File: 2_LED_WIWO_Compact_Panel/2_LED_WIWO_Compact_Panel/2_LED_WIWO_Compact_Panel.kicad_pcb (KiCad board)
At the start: 2 copper layers, 77.5 x 56.5 mm, 77 parts, among them J3 Screw_Terminal_01x03, J4 Screw_Terminal_01x03, Q1 AO3400A, U1 AP2210N-5.0TRG1, U2 XL1509, U3 NE555DR-EV, U4 NE555DR-EV, U5 MP24833-AGN-Z, U6 MP24833-AGN-Z

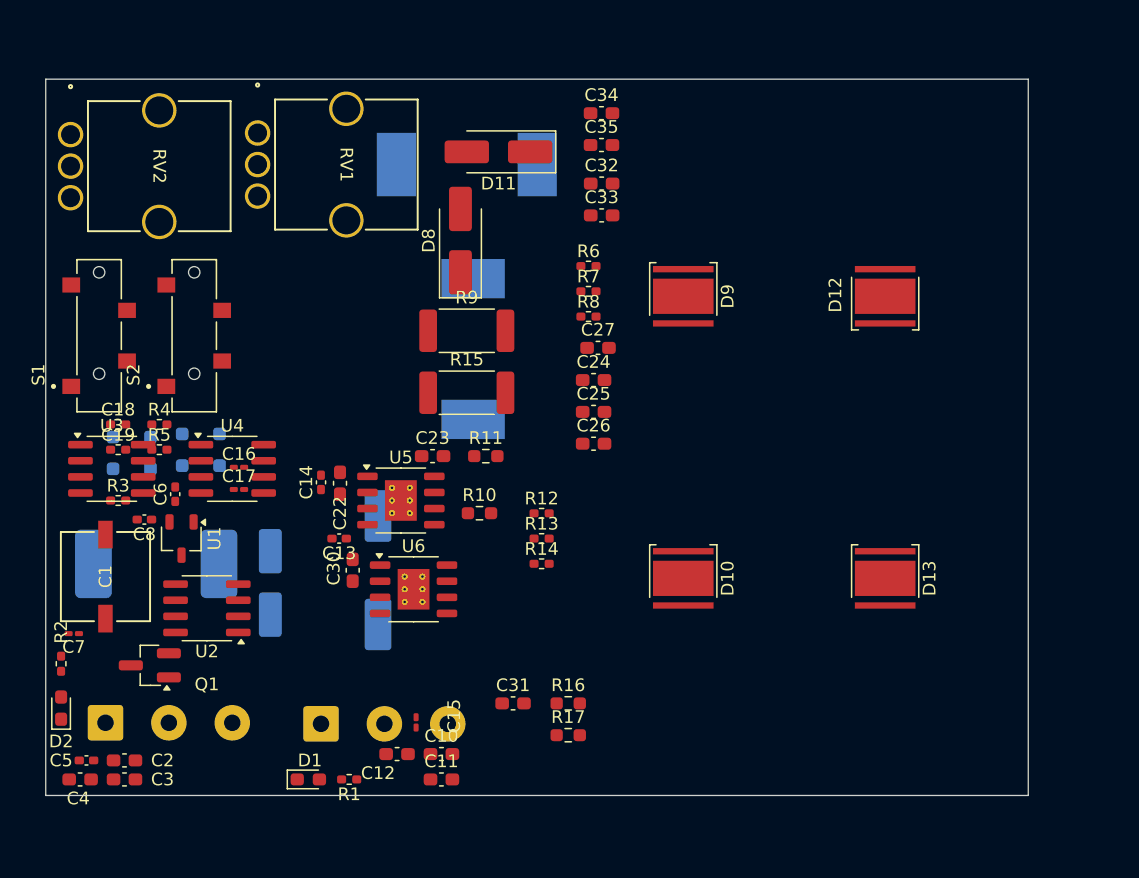
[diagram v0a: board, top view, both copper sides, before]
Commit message: v1 route done
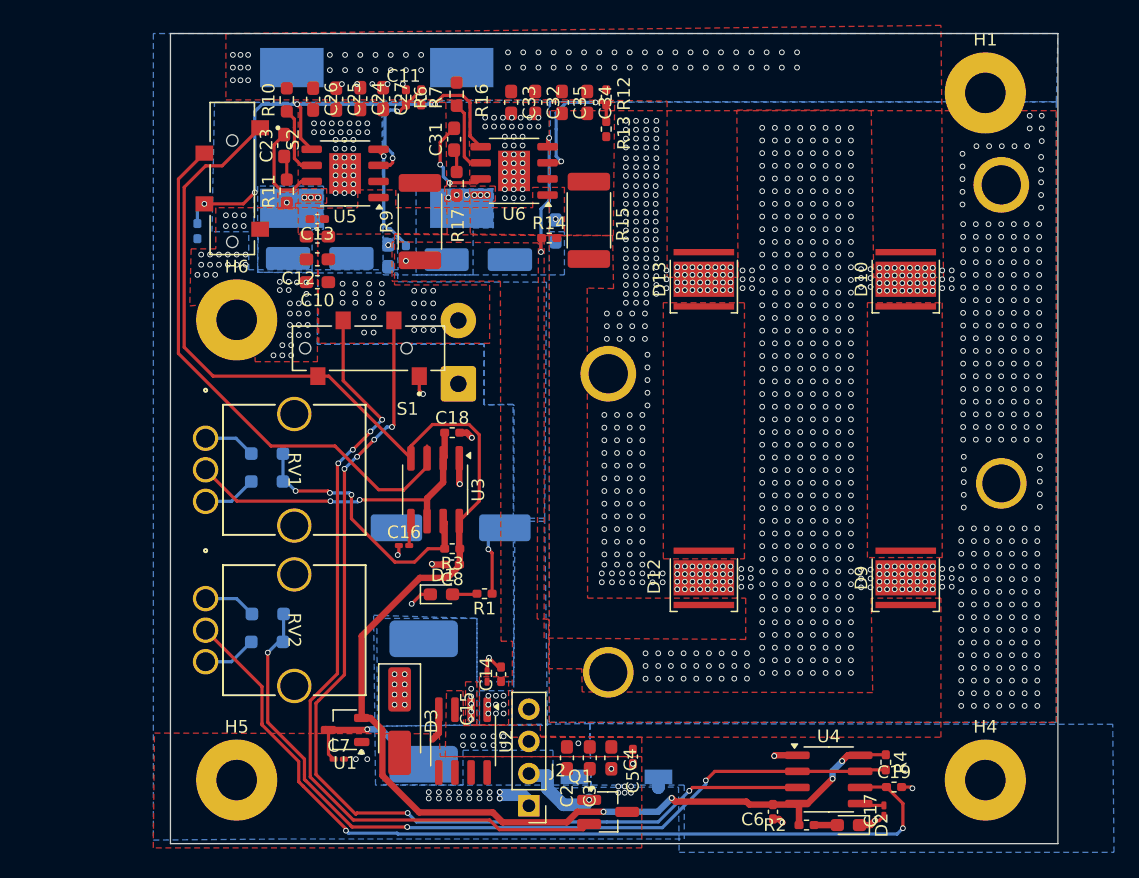
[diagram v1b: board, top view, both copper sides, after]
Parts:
- removed J3, J4: Screw_Terminal_01x03, TerminalBlock:TerminalBlock_MaiXu_MX126-5.0-03P_1x03_P5.00mm
- added E1: ~, heatsinks:small_heatsink, B.Cu at (183.7, 71.5)
- added E2: ~, heatsinks:small_heatsink, B.Cu at (183.7, 95.1)
- added H1: MountingHole_Pad, MountingHole:MountingHole_3.2mm_M3_Pad, F.Cu at (197.9, 56.9)
- added H4: MountingHole_Pad, MountingHole:MountingHole_3.2mm_M3_Pad, F.Cu at (197.9, 111.0)
- added H5: MountingHole_Pad, MountingHole:MountingHole_3.2mm_M3_Pad, F.Cu at (138.8, 111.0)
- added H6: MountingHole_Pad, MountingHole:MountingHole_3.2mm_M3_Pad, F.Cu at (138.8, 74.8)
- added J1: Screw_Terminal_01x02, TerminalBlock:TerminalBlock_MaiXu_MX126-5.0-02P_1x02_P5.00mm, B.Cu at (156.3, 79.8)
- added J2: Conn_01x04_Pin, Connector_PinHeader_2.54mm:PinHeader_1x04_P2.54mm_Vertical, F.Cu at (161.9, 113.1)
- C1, C22, C30, D11, D8, R5, R8: moved to B.Cu
- D3: moved to F.Cu
- moved C19 66.7 mm to (190.7, 111.6)
- moved R4 63.2 mm to (190.1, 109.7), turned to -90 degrees
- moved D2 62.8 mm to (187.1, 114.6), turned to 180 degrees
- moved R2 60.2 mm to (183.8, 114.6), turned to 0 degrees
- moved C17 56.8 mm to (189.9, 113.5), turned to 90 degrees
- moved C6 53.4 mm to (181.2, 113.5), turned to -90 degrees
- moved U4 53.0 mm to (185.6, 111.0)
- moved R16 48.8 mm to (156.2, 57.0), turned to 90 degrees
- moved C31 44.7 mm to (156.0, 60.5), turned to 90 degrees
- moved R17 44.4 mm to (156.2, 64.0), turned to 90 degrees
- moved C11 43.9 mm to (145.2, 68.2), turned to 180 degrees
- moved C1 43.3 mm to (168.8, 110.8), turned to 0 degrees
- moved C5 43.1 mm to (170.1, 109.2), turned to -90 degrees
- moved C4 41.9 mm to (168.4, 109.3), turned to -90 degrees
- moved C12 39.5 mm to (145.2, 70.0)
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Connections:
- C18 pad 1: /TR_THR -> /LED_TR_THR
- C19 pad 1: /TR_THR -> /FAN_TR_THR
- C22 pad 2: PGND -> PGND_1
- C24 pad 2: PGND -> PGND_1
- C25 pad 2: PGND -> PGND_1
- C26 pad 2: PGND -> PGND_1
- C27 pad 2: PGND -> PGND_1
- C30 pad 2: PGND -> PGND_2
- C32 pad 2: PGND -> PGND_2
- C33 pad 2: PGND -> PGND_2
- C34 pad 2: PGND -> PGND_2
- C35 pad 2: PGND -> PGND_2
- D11 pad 2: PGND -> PGND_2
- D4 pad 2: /DIS -> /LED_DIS
- D5 pad 2: /DIS -> /FAN_DIS
- D6 pad 1: /DIS -> /LED_DIS
- D7 pad 1: /DIS -> /FAN_DIS
- D8 pad 2: PGND -> PGND_1
- R13 pad 2: PGND -> PGND_2
- R15 pad 2: PGND -> PGND_2
- R3 pad 2: /DIS -> /LED_DIS
- R4 pad 2: /DIS -> /FAN_DIS
- R7 pad 2: PGND -> PGND_1
- R9 pad 2: PGND -> PGND_1
- RV1 pad 2: /TR_THR -> /LED_TR_THR
- RV2 pad 2: /TR_THR -> /FAN_TR_THR
- U3 pad 2: /TR_THR -> /LED_TR_THR
- U3 pad 6: /TR_THR -> /LED_TR_THR
- U3 pad 7: /DIS -> /LED_DIS
- U4 pad 2: /TR_THR -> /FAN_DIS
- U4 pad 6: /TR_THR -> /FAN_TR_THR
- U4 pad 7: /DIS -> /FAN_DIS
- U5 pad 2: PGND -> PGND_1
- U5 pad 9: PGND -> PGND_1
- U6 pad 2: PGND -> PGND_2
- U6 pad 9: PGND -> PGND_2
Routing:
- net +5V: track 0.00 -> 128.6 mm, vias 0 -> 4
- net /FAN_PWM: track 0.00 -> 79.4 mm, vias 0 -> 6
- net /FAN_TR_THR: track 0.00 -> 70.5 mm, vias 0 -> 2
- net /FAN_DIS: track 0.00 -> 64.5 mm, vias 0 -> 3
- net Net-(Q1-G): track 0.00 -> 63.6 mm, vias 0 -> 4
- net /LED_PWM: track 0.00 -> 43.1 mm
- net /LED_EN: track 0.00 -> 38.1 mm, vias 0 -> 4
- net GND: track 0.00 -> 26.8 mm, vias 0 -> 151
- net /LED_TR_THR: track 0.00 -> 26.2 mm, vias 0 -> 2
- net /LED_DIS: track 0.00 -> 22.3 mm, vias 0 -> 3
- net /FB_2: track 0.00 -> 11.1 mm, vias 0 -> 2
- net /OVP_2: track 0.00 -> 11.0 mm, vias 0 -> 2
- net /OVP_1: track 0.00 -> 8.96 mm, vias 0 -> 2
- net /FB_1: track 0.00 -> 8.62 mm, vias 0 -> 1
- net +12V: track 0.00 -> 8.14 mm, vias 0 -> 12
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- added copper zone on B.Cu, net +12V
- added copper zone on F.Cu, net +12V
- added copper zone on B.Cu, net /LED_EPAD
- added copper zone on F.Cu, net /LED_EPAD
- added copper zone on B.Cu, net /SW_1
- added copper zone on F.Cu, net /SW_1
- added copper zone on B.Cu, net /SW_2
- added copper zone on F.Cu, net /SW_2
- added copper zone on F.Cu, net /VLED_1_n
- added copper zone on F.Cu, net /VLED_2_n
- added copper zone on B.Cu, net GND
- added copper zone on F.Cu, net GND
- added copper zone on F.Cu, net Net-(D10-K)
- added copper zone on F.Cu, net Net-(D12-A)
- added copper zone on B.Cu, net Net-(D3-K)
- added copper zone on F.Cu, net Net-(D3-K)
- added copper zone on B.Cu, net PGND_1
- added copper zone on F.Cu, net PGND_1
- added copper zone on B.Cu, net PGND_2
- added copper zone on F.Cu, net PGND_2
- added copper zone on B.Cu, net VCC
- added copper zone on F.Cu, net VCC
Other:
- board size 77.5 x 56.5 mm -> 70 x 63.9 mm
